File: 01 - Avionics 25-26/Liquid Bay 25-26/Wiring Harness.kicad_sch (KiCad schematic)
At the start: 1 part, among them J2 M12A-08PMMP-SF8001

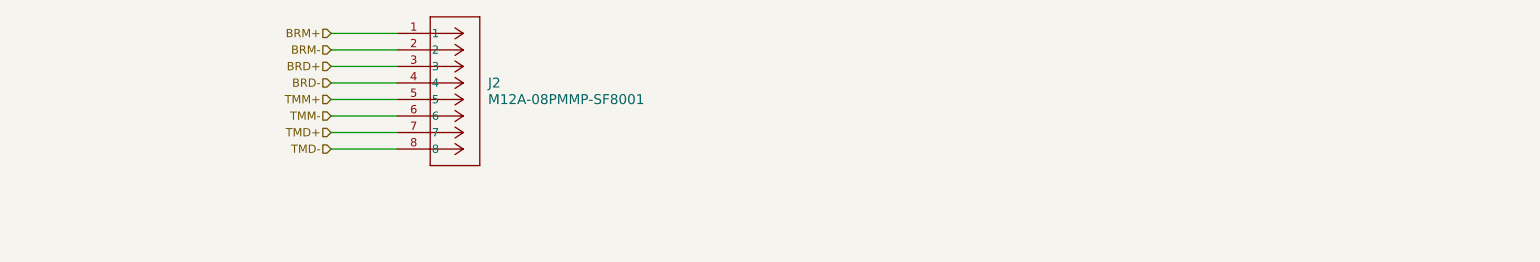
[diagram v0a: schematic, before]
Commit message: Add files via upload
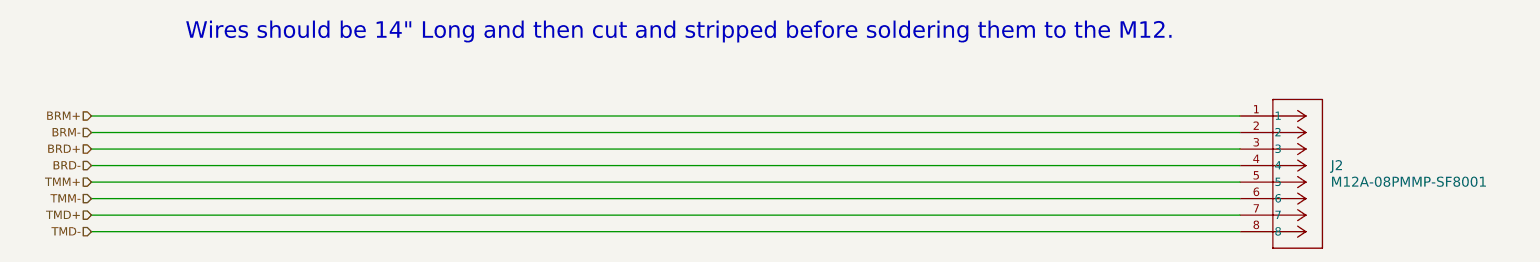
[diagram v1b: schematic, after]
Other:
- note added: "Wires should be 14" Long and then cut and stripped before soldering them to the M12."
- moved on the sheet: J2
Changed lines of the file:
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@@
 	(title_block
 		(title "Liquid Project Avionics Bay Wiring")
-		(date "2025-10-10")
+		(date "2025-10-11")
 		(rev "IR")
 		(company "Missouri S&T Rocket Design Team")
 		(comment 1 "Author(s): Isaac Lough")
 	)
-	(wire
-		(pts
-			(xy 90.17 81.28) (xy 100.33 81.28)
-		)
-		(stroke
-			(width 0)
-			(type default)
-		)
-	)
-	(wire
-		(pts
-			(xy 90.17 93.98) (xy 100.33 93.98)
-		)
-		(stroke
-			(width 0)
-			(type default)
-		)
-	)
-	(wire
-		(pts
-			(xy 90.17 88.9) (xy 100.33 88.9)
-		)
-		(stroke
-			(width 0)
-			(type default)
-		)
-	)
-	(wire
-		(pts
-			(xy 90.17 99.06) (xy 100.33 99.06)
-		)
-		(stroke
-			(width 0)
-			(type default)
-		)
-	)
-	(wire
-		(pts
-			(xy 90.17 91.44) (xy 100.33 91.44)
-		)
-		(stroke
-			(width 0)
-			(type default)
-		)
-	)
-	(wire
-		(pts
-			(xy 90.17 83.82) (xy 100.33 83.82)
-		)
-		(stroke
-			(width 0)
-			(type default)
-		)
-	)
-	(wire
-		(pts
-			(xy 90.17 86.36) (xy 100.33 86.36)
-		)
-		(stroke
-			(width 0)
-			(type default)
-		)
-	)
-	(wire
-		(pts
-			(xy 90.17 96.52) (xy 100.33 96.52)
+	(text "Wires should be 14\" Long and then cut and stripped before soldering them to the M12. "
+		(exclude_from_sim no)
+		(at 143.764 81.026 0)
+		(effects
+			(font
+				(size 2.54 2.54)
+			)
+		)
+	)
+	(wire
+		(pts
+			(xy 53.34 93.98) (xy 229.87 93.98)
+		)
+		(stroke
+			(width 0)
+			(type default)
+		)
+	)
+	(wire
+		(pts
+			(xy 53.34 106.68) (xy 229.87 106.68)
+		)
+		(stroke
+			(width 0)
+			(type default)
+		)
+	)
+	(wire
+		(pts
+			(xy 53.34 101.6) (xy 229.87 101.6)
+		)
+		(stroke
+			(width 0)
+			(type default)
+		)
+	)
+	(wire
+		(pts
+			(xy 53.34 111.76) (xy 229.87 111.76)
+		)
+		(stroke
+			(width 0)
+			(type default)
+		)
+	)
+	(wire
+		(pts
+			(xy 53.34 104.14) (xy 229.87 104.14)
+		)
+		(stroke
+			(width 0)
+			(type default)
+		)
+	)
+	(wire
+		(pts
+			(xy 53.34 96.52) (xy 229.87 96.52)
+		)
+		(stroke
+			(width 0)
+			(type default)
+		)
+	)
+	(wire
+		(pts
+			(xy 53.34 99.06) (xy 229.87 99.06)
+		)
+		(stroke
+			(width 0)
+			(type default)
+		)
+	)
+	(wire
+		(pts
+			(xy 53.34 109.22) (xy 229.87 109.22)
 		)
 		(stroke
@@
 	(hierarchical_label "BRM+"
 		(shape input)
-		(at 90.17 81.28 180)
+		(at 53.34 93.98 180)
 		(effects
 			(font
@@
 	(hierarchical_label "TMM+"
 		(shape input)
-		(at 90.17 91.44 180)
+		(at 53.34 104.14 180)
 		(effects
 			(font
@@
 	(hierarchical_label "TMD+"
 		(shape input)
-		(at 90.17 96.52 180)
+		(at 53.34 109.22 180)
 		(effects
 			(font
@@
 	(hierarchical_label "TMD-"
 		(shape input)
-		(at 90.17 99.06 180)
+		(at 53.34 111.76 180)
 		(effects
 			(font
@@
 	(hierarchical_label "BRM-"
 		(shape input)
-		(at 90.17 83.82 180)
+		(at 53.34 96.52 180)
 		(effects
 			(font
@@
 	(hierarchical_label "TMM-"
 		(shape input)
-		(at 90.17 93.98 180)
+		(at 53.34 106.68 180)
 		(effects
 			(font
@@
 	(hierarchical_label "BRD-"
 		(shape input)
-		(at 90.17 88.9 180)
+		(at 53.34 101.6 180)
 		(effects
 			(font
@@
 	(hierarchical_label "BRD+"
 		(shape input)
-		(at 90.17 86.36 180)
+		(at 53.34 99.06 180)
 		(effects
 			(font
@@
 	(symbol
 		(lib_id "2601-3108:M12A-08PMMP-SF8001")
-		(at 100.33 81.28 0)
+		(at 229.87 93.98 0)
 		(unit 1)
 		(exclude_from_sim no)
@@
 		(fields_autoplaced yes)
 		(property "Reference" "J2"
-			(at 114.3 88.8999 0)
+			(at 243.84 101.5999 0)
 			(effects
 				(font
@@
 		)
 		(property "Value" "M12A-08PMMP-SF8001"
-			(at 114.3 91.4399 0)
+			(at 243.84 104.1399 0)
 			(effects
 				(font
@@
 		)
 		(property "Footprint" "CONN_M12A-08PMMP-SF8001_AMP"
-			(at 100.33 81.28 0)
+			(at 229.87 93.98 0)
 			(effects
 				(font
@@
 		)
 		(property "Datasheet" "M12A-08PMMP-SF8001"
-			(at 100.33 81.28 0)
+			(at 229.87 93.98 0)
 			(effects
 				(font
@@
 		)
 		(property "Description" ""
-			(at 100.33 81.28 0)
-			(effects
-				(font
+			(at 229.87 93.98 0)
+			(effects
+				(font
